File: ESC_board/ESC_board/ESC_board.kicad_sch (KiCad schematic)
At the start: 1 part

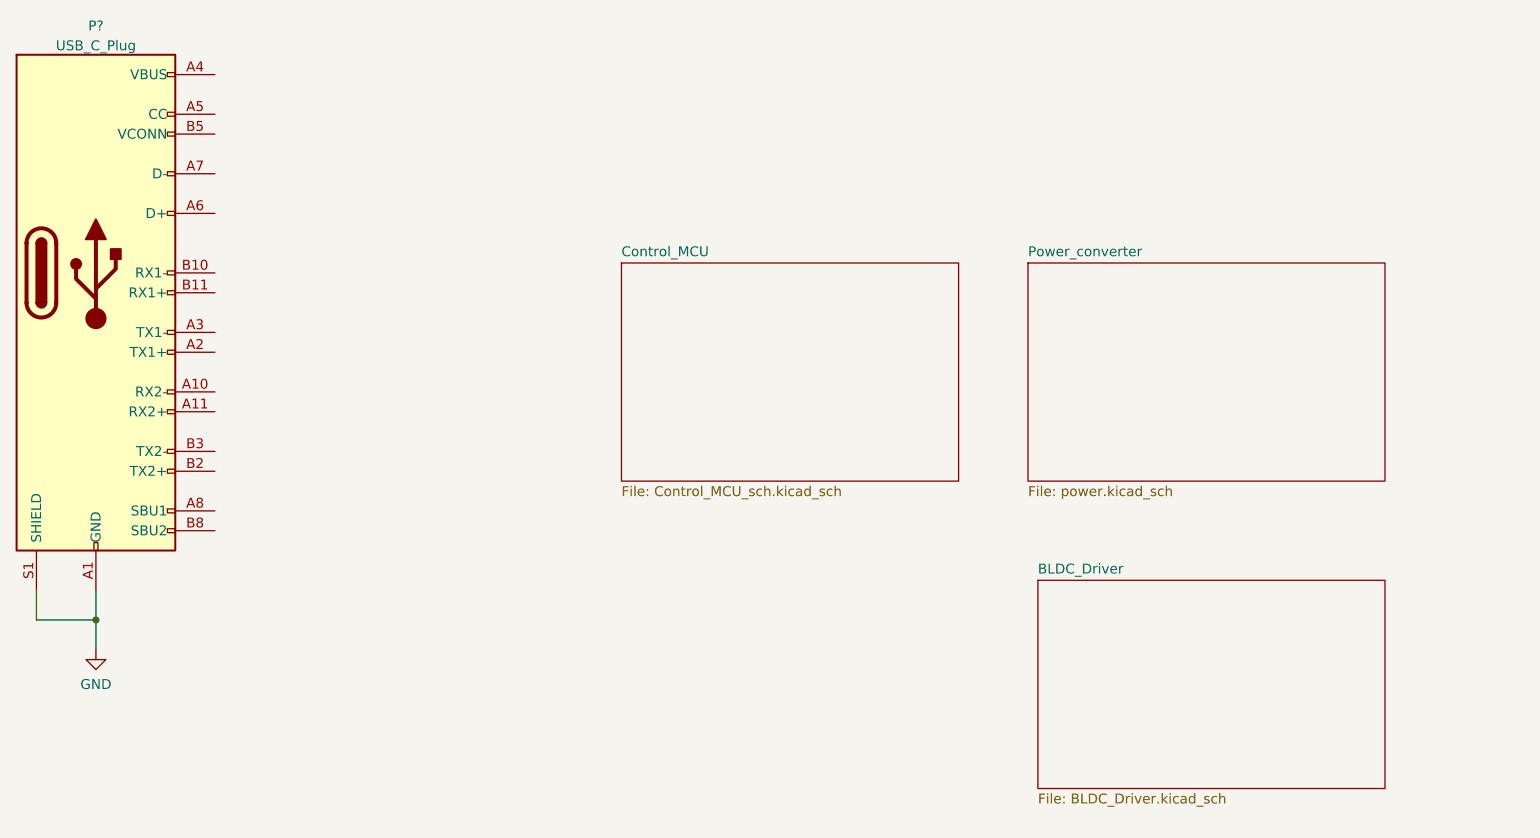
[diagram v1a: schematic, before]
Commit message: Updated localization files
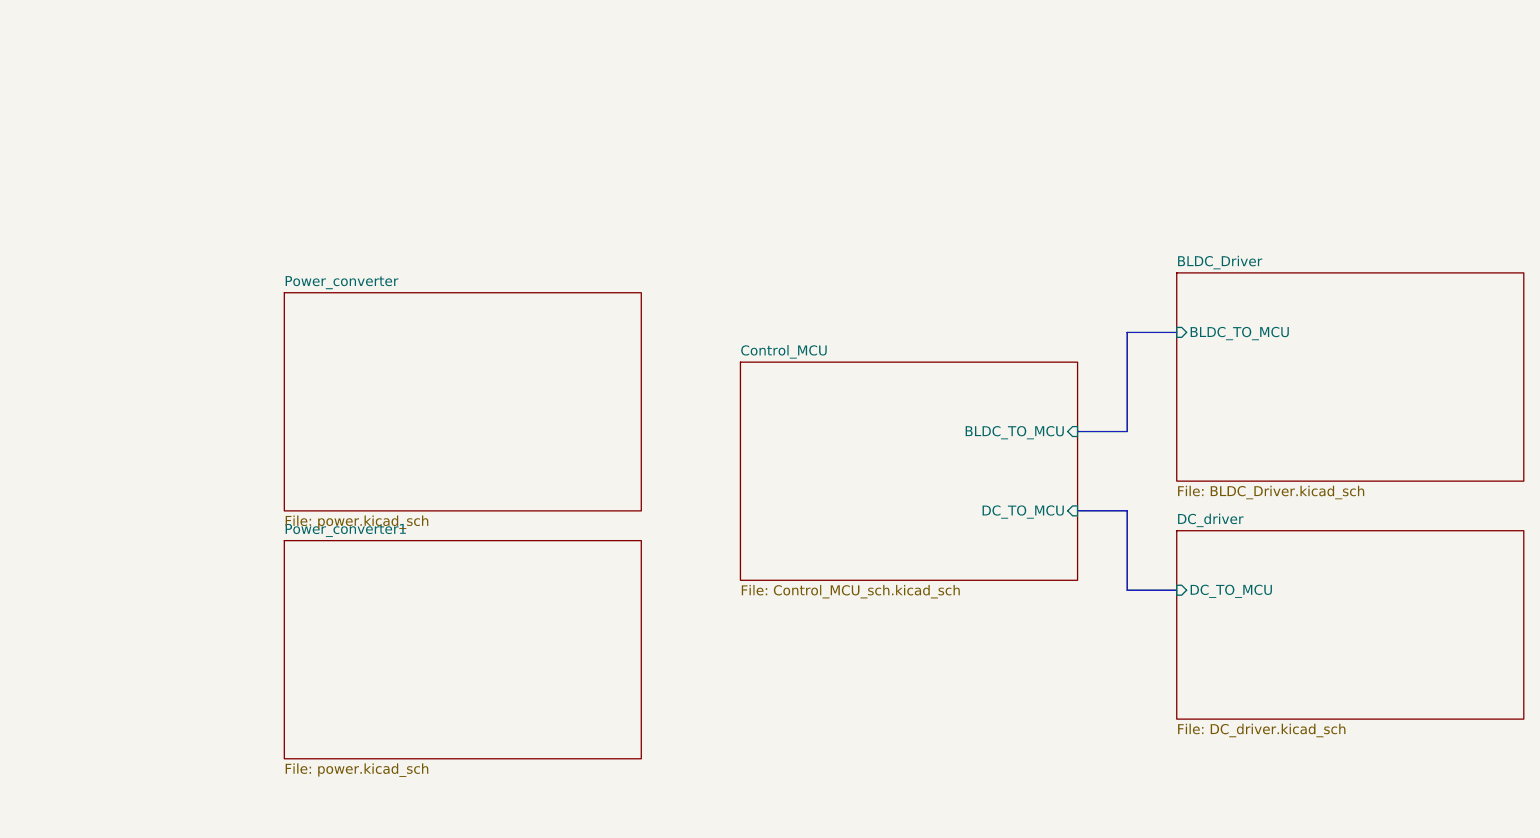
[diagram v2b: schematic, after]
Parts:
- removed P?: USB_C_Plug, symbol Connector:USB_C_Plug
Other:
- added sheet DC_driver (DC_driver.kicad_sch)
- added sheet Power_converter1 (power.kicad_sch)
- sheet BLDC_Driver ports: added BLDC_TO_MCU; removed none
- sheet Control_MCU ports: added BLDC_TO_MCU, DC_TO_MCU; removed none

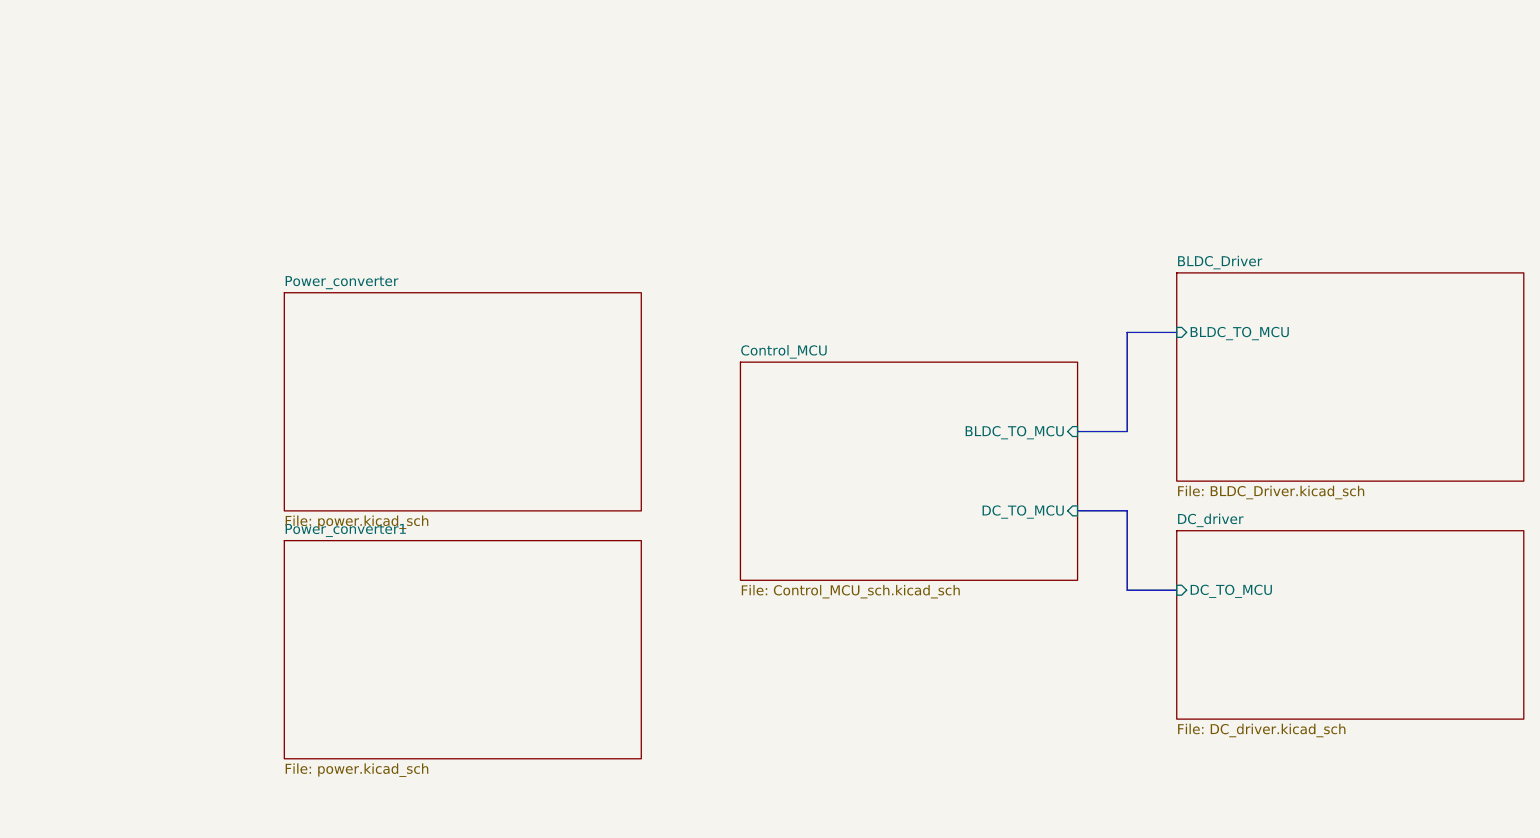
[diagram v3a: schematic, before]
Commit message: Added ESC schematic and board layout
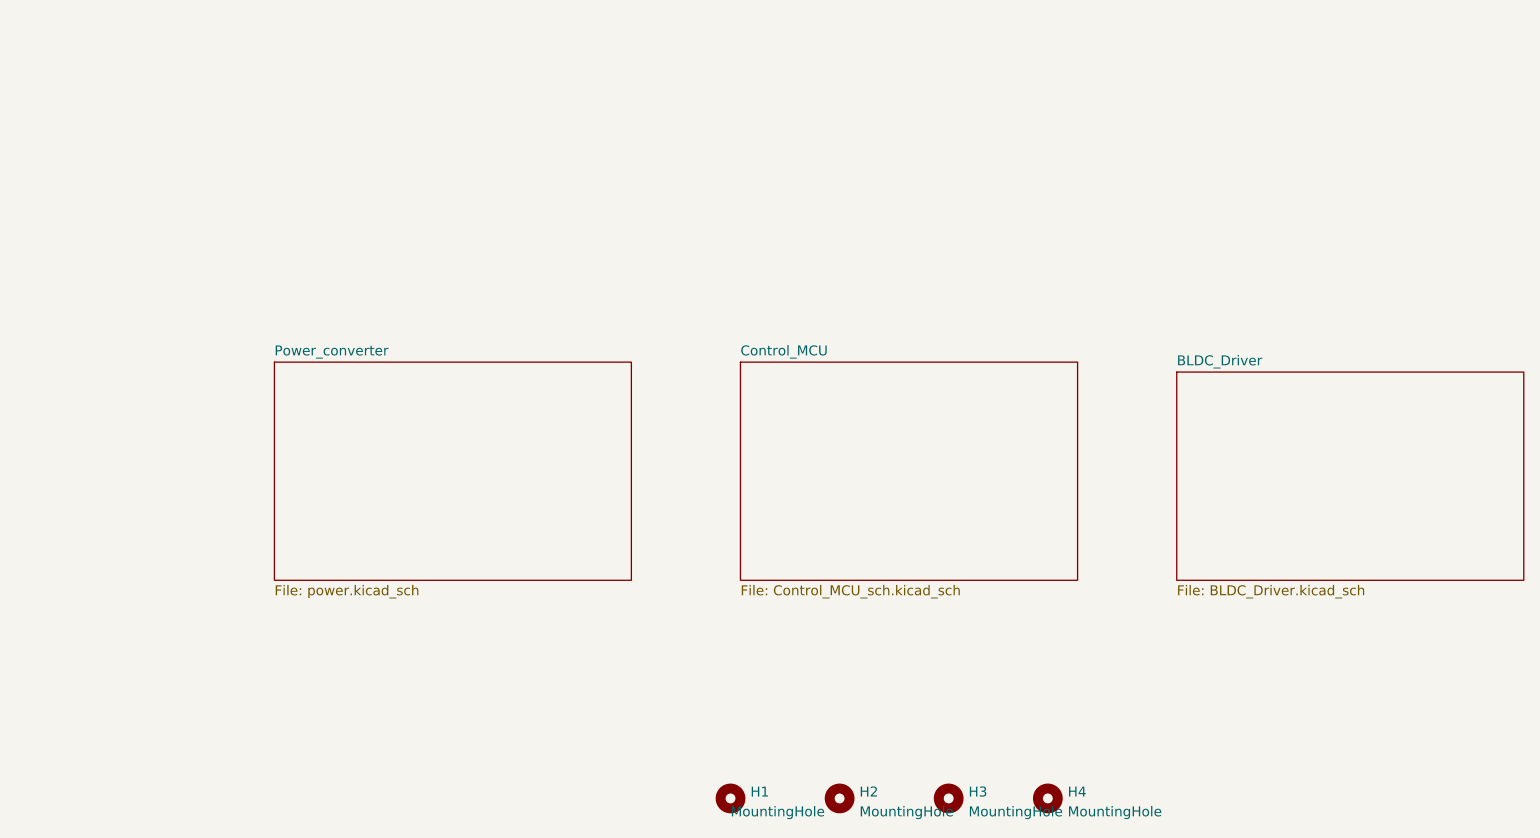
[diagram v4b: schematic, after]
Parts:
- added H1, H2, H3, H4: MountingHole, MountingHole:MountingHole_2.2mm_M2_Pad_Via, symbol Mechanical:MountingHole
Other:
- removed sheet DC_driver
- removed sheet Power_converter1
- sheet BLDC_Driver ports: added none; removed BLDC_TO_MCU
- sheet Control_MCU ports: added none; removed BLDC_TO_MCU, DC_TO_MCU
